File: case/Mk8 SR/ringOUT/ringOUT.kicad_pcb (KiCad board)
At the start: 2 copper layers, 44 x 43.6 mm, 1 part

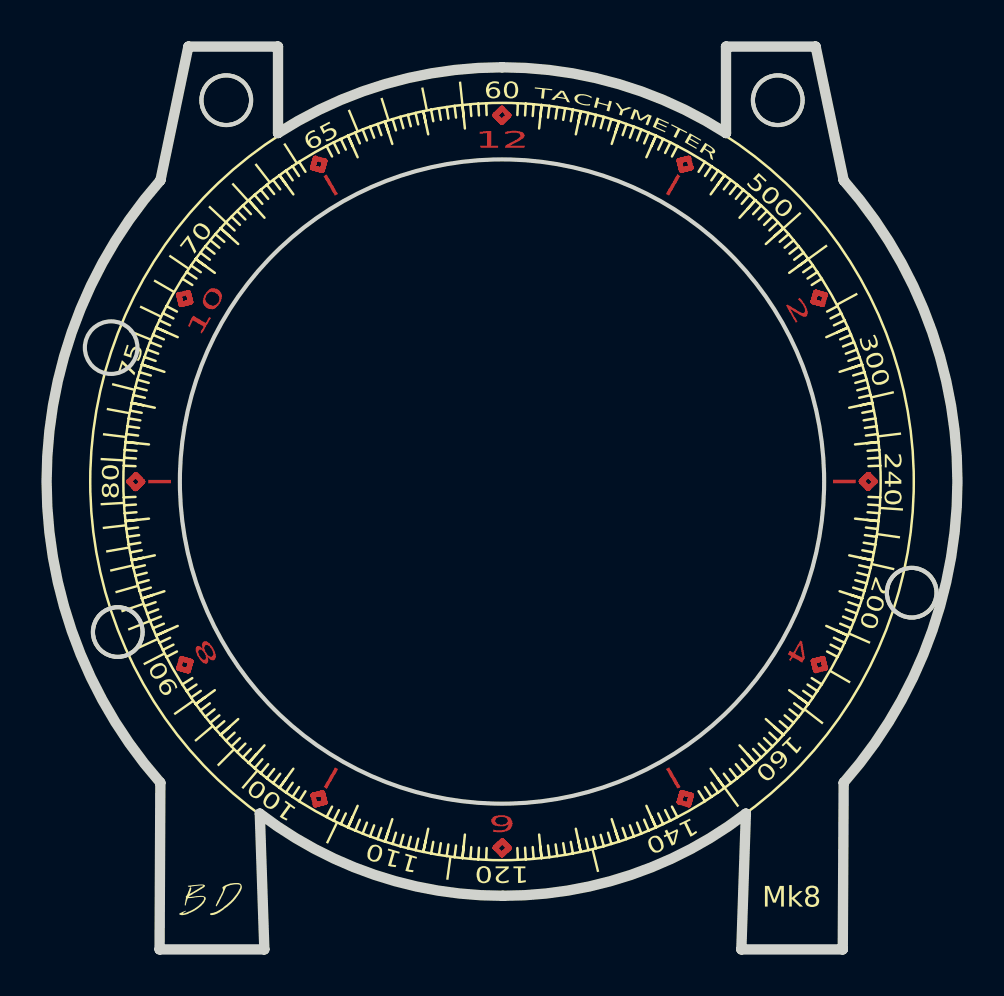
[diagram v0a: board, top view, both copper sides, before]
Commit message: new ring
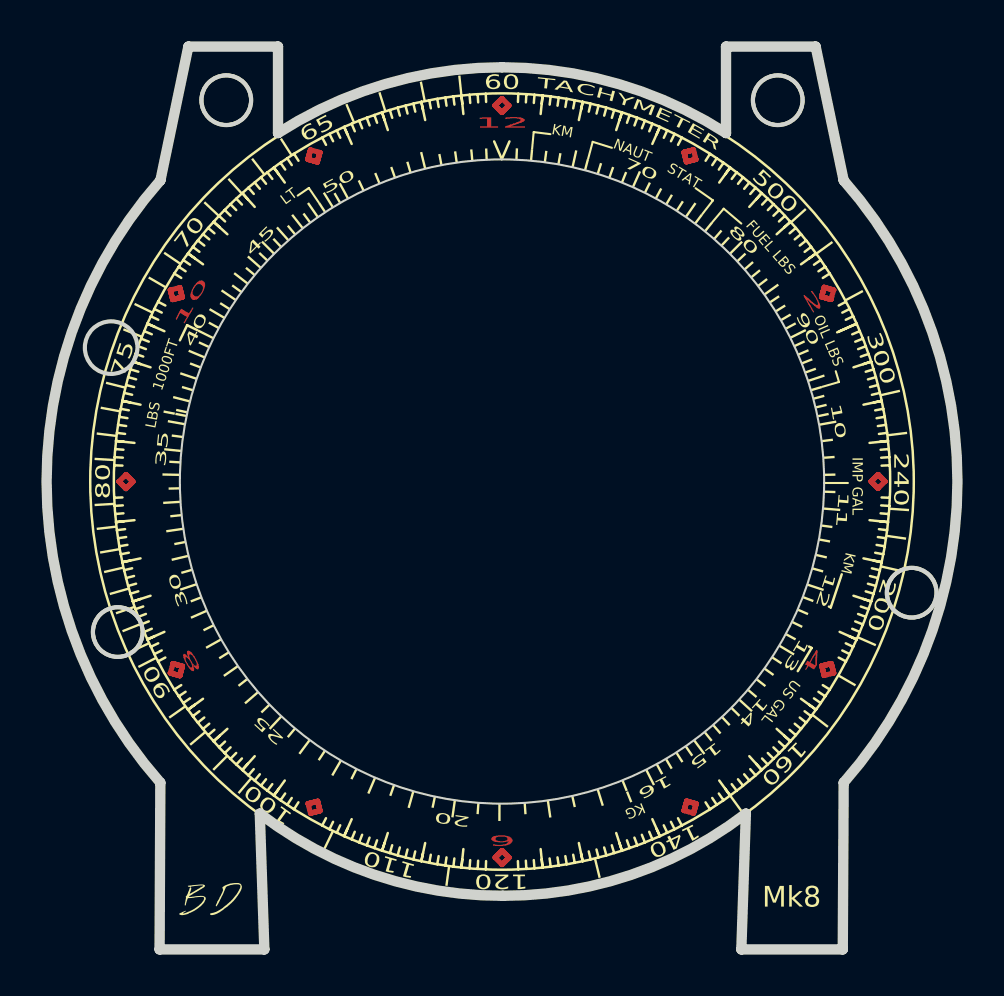
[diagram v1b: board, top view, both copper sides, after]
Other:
- board text added: "1000FT"
- board text added: "11"
- board text added: "13"
- board text added: "14"
- board text added: "15"
- board text added: "16"
- board text added: "20"
- board text added: "25"
- board text added: "30"
- board text added: "35"
- board text added: "40"
- board text added: "45"
- board text added: "50"
- board text added: "FUEL LBS"
- board text added: "IMP GAL"
- board text added: "KG"
- board text added: "KM"
- board text added: "LBS"
- board text added: "LT"
- board text added: "NAUT"
- board text added: "OIL LBS"
- board text added: "STAT"
- board text added: "US GAL"
